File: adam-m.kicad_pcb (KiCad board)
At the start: 2 copper layers, 114.5 x 95.3 mm, 21 parts, among them J1 AudioJack4dpb, SW1 SW_Push, SW10 SW_Push, SW11 SW_Push, SW12 SW_Push, SW13 SW_Push, SW14 SW_Push, SW15 SW_Push, SW16 SW_Push, SW17 SW_Push, SW2 SW_Push, SW3 SW_Push, SW4 SW_Push, SW5 SW_Push, SW6 SW_Push, SW7 SW_Push, SW8 SW_Push, SW9 SW_Push, U1 ProMicro-kbd

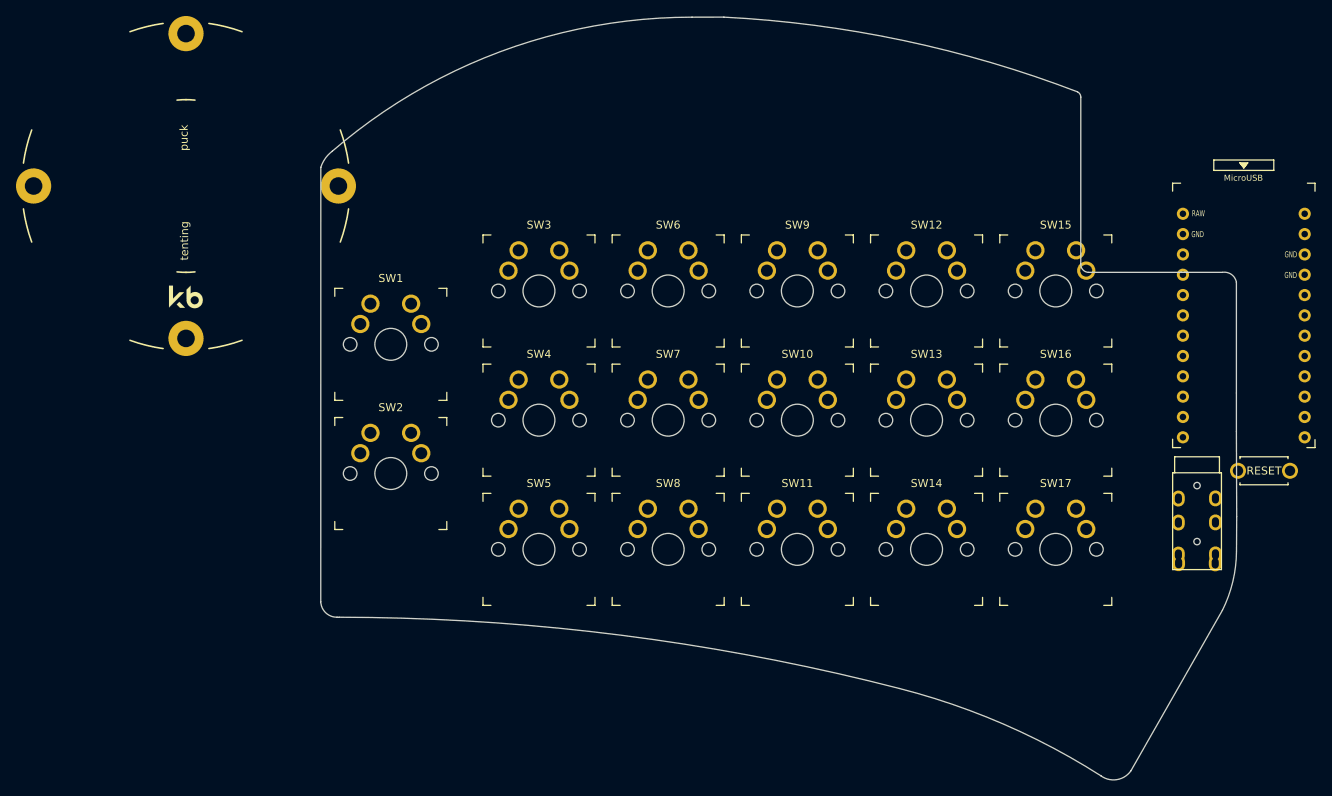
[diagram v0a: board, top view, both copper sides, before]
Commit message: some poc routing
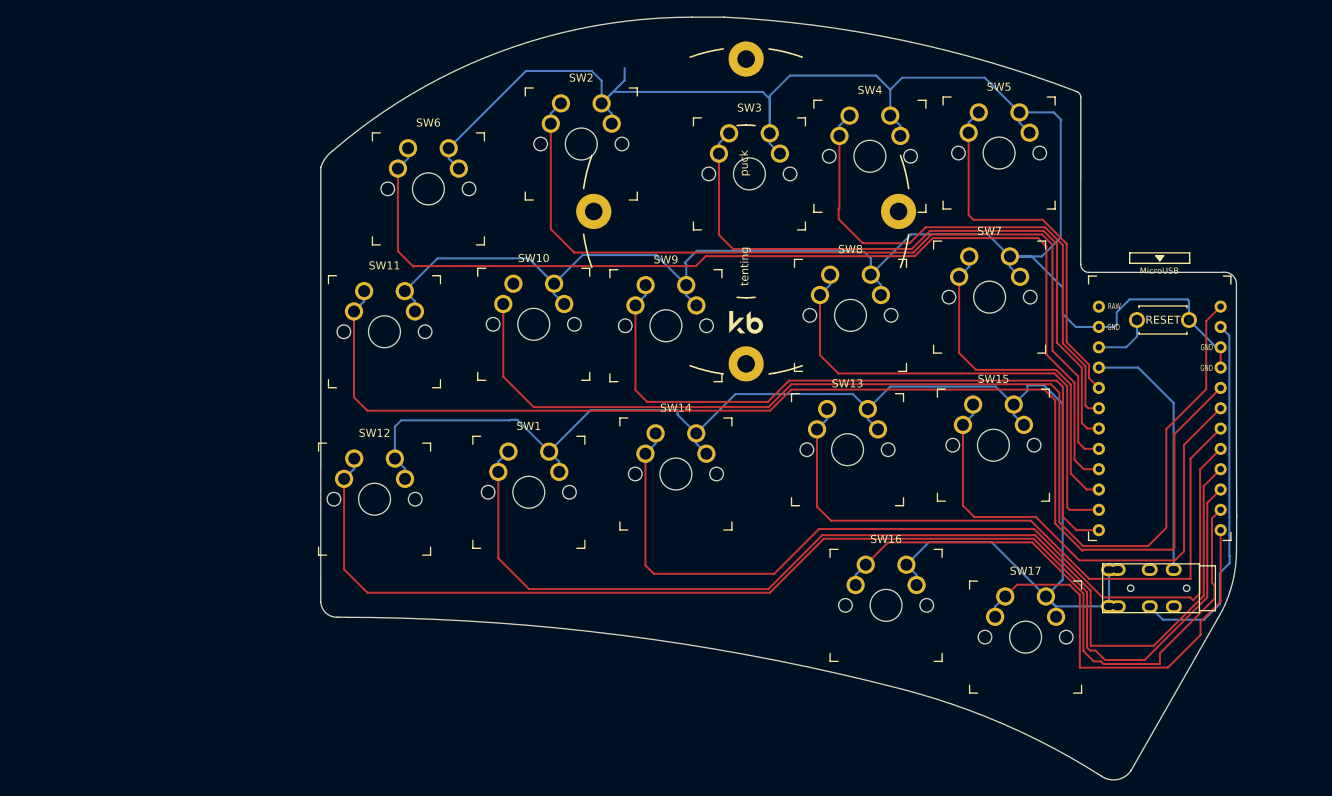
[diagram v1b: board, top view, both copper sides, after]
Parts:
- moved SW5 75.9 mm to (190.4, 47.9)
- moved SW12 73.7 mm to (112.3, 91.1)
- moved H1 70.1 mm to (158.8, 55.2)
- moved SW11 58.3 mm to (113.6, 70.2)
- moved SW4 52.9 mm to (174.3, 48.3)
- moved SW2 47.6 mm to (138.2, 46.7)
- moved SW7 43.0 mm to (189.2, 65.9)
- moved SW8 37.1 mm to (171.8, 68.2)
- moved SW10 35.1 mm to (132.2, 69.3)
- moved SW14 32.7 mm to (150.0, 88.0)
- moved SW6 32.6 mm to (119.1, 52.4)
- moved SW16 31.4 mm to (176.3, 104.4)
- moved SW3 30.1 mm to (159.2, 50.5)
- moved SW1 25.3 mm to (131.6, 90.3)
- moved RSW1 22.7 mm to (210.9, 68.7)
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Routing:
- net gnd: track 0.00 -> 474.2 mm
- net Switch11: track 0.00 -> 158.0 mm
- net Switch15: track 0.00 -> 154.0 mm
- net Switch10: track 0.00 -> 144.0 mm
- net Switch1: track 0.00 -> 135.5 mm
- net Switch6: track 0.00 -> 128.8 mm
- net Switch14: track 0.00 -> 112.3 mm
- net Switch2: track 0.00 -> 110.6 mm
- net Switch9: track 0.00 -> 90.5 mm
- net Switch3: track 0.00 -> 83.9 mm
- net Switch13: track 0.00 -> 83.5 mm
- net Switch16: track 0.00 -> 74.2 mm
- net Switch4: track 0.00 -> 67.6 mm
- net Switch12: track 0.00 -> 63.9 mm
- net Switch8: track 0.00 -> 62.3 mm
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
